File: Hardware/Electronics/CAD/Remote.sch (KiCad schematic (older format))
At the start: 47 parts, among them J1 CONN_01X12, J2 CONN_01X03, J3 CONN_01X05, J4 CONN_01X01, J5 CONN_01X01, J6 CONN_01X24, Q1 AO3418, Q2 Q_NPN_BCE, SW1 SW_DPST_x2, U2 MCP23S17, U3 ESP-12E, U4 LD1117S33CTR

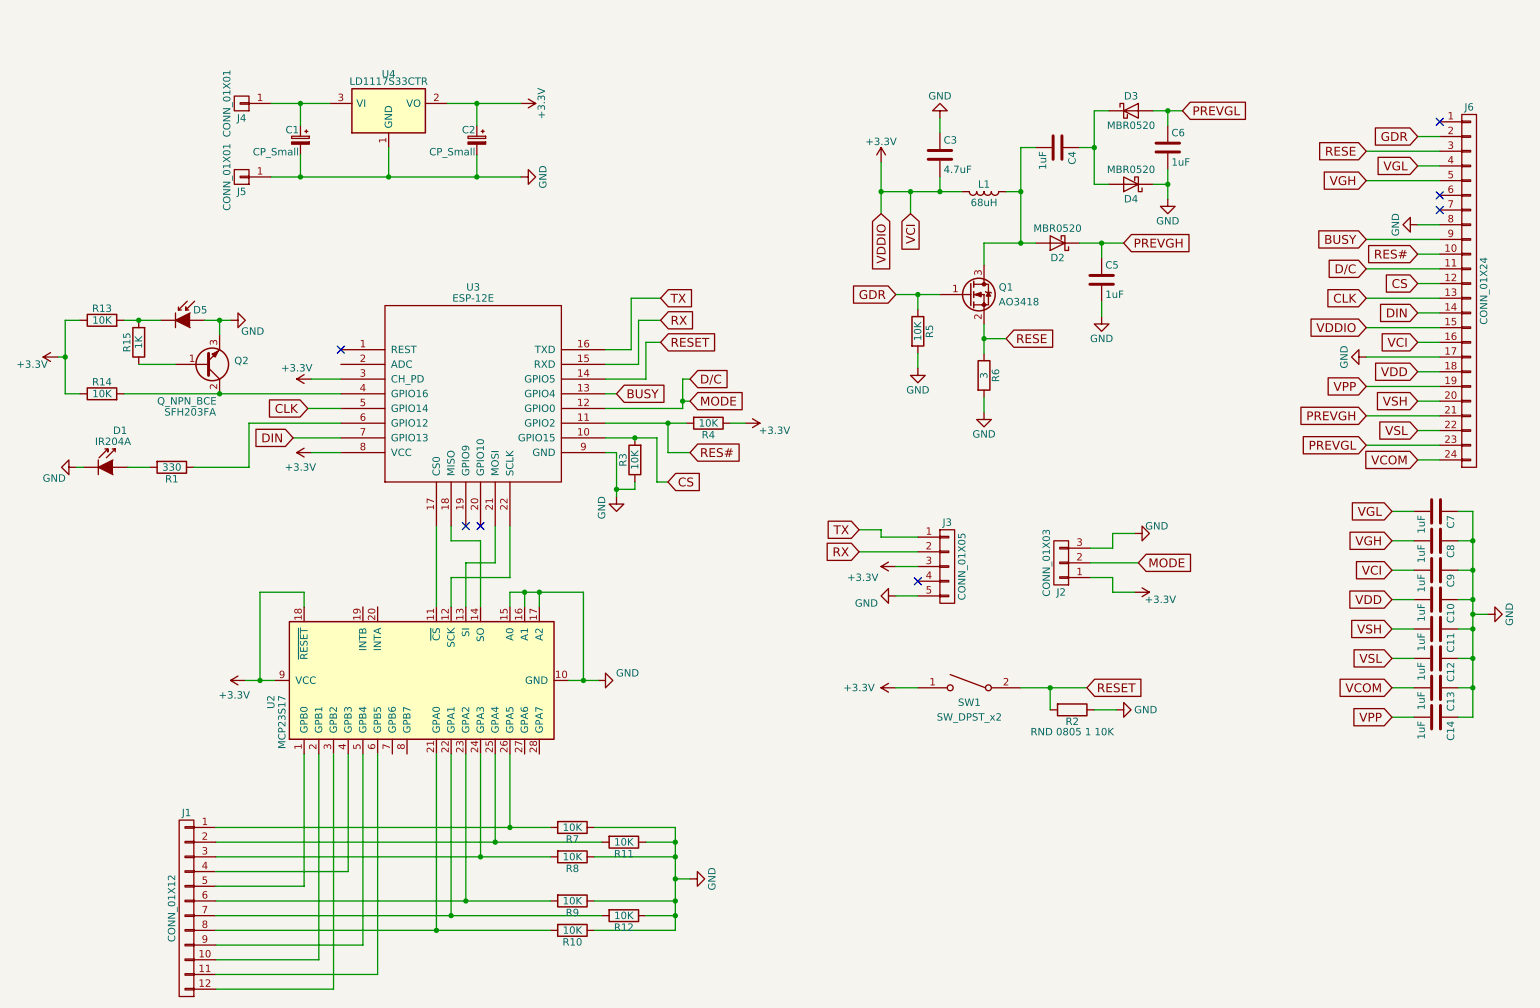
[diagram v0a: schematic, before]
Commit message: update design
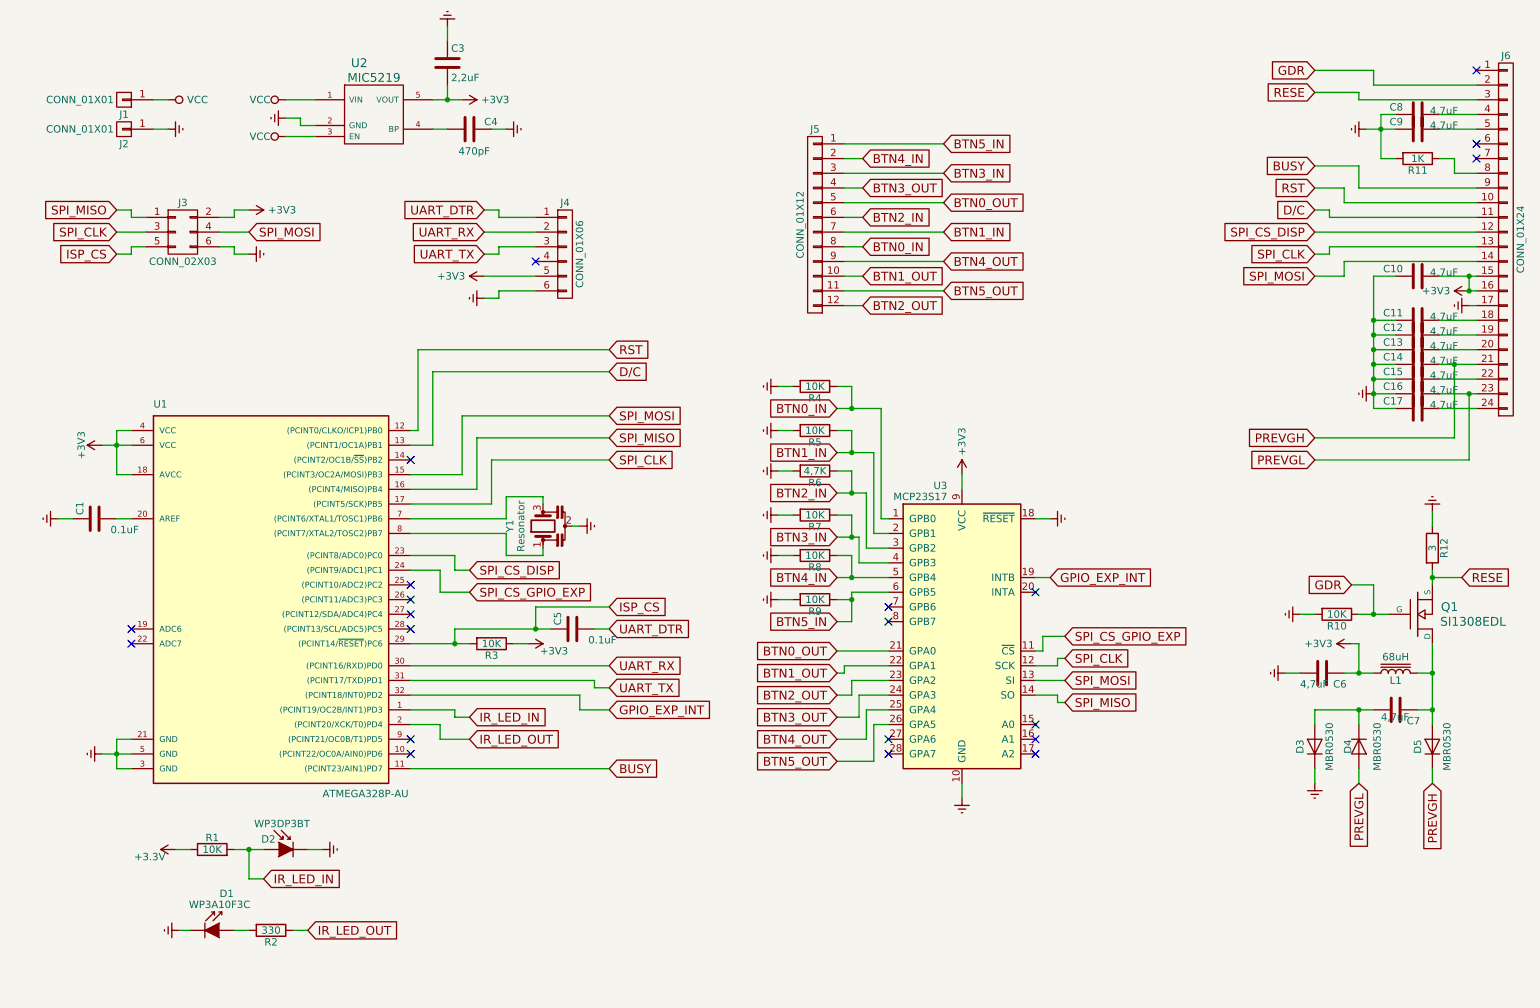
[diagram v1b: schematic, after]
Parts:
- removed C1, C2: CP_Small, Capacitor:CP_8x11.5mm_hor, symbol CP_Small
- removed D2, D3, D4: MBR0520, Diodes_SMD:D_SOD-123, symbol D_Schottky
- removed J2: CONN_01X03, Terminal:Pin_Header_SMD_1x3_Angled_2.54mm, symbol CONN_01X03
- removed J3: CONN_01X05, Terminal:SolderPad_1x5_3.81mm, symbol CONN_01X05
- removed L1: 68uH, Inductors_SMD:L_0805, symbol L
- removed Q1: AO3418, TO_SOT_Packages_SMD:SOT-23, symbol Q_NMOS_GSD
- removed Q2: Q_NPN_BCE, TO_SOT_Packages_SMD:SOT-23, symbol Q_NPN_BCE
- removed R14: 10K, Resistors_SMD:R_0805, symbol R
- removed R15: 1K, Resistors_SMD:R_0805, symbol R
- removed R2: RND 0805 1 10K, Resistors_SMD:R_0805, symbol R
- removed SW1: SW_DPST_x2, Buttons_Switches_SMD:SW_SPST_SKQG, symbol SW_DPST_x2
- removed U2: MCP23S17, Housings_SOIC:SOIC-28W_7.5x17.9mm_Pitch1.27mm, symbol MCP23S17
- removed U3: ESP-12E, ESP8266:ESP-12E_SMD, symbol ESP-12E
- removed U4: LD1117S33CTR, TO_SOT_Packages_SMD:SOT-223, symbol LD1117S33CTR
- added C1: 0.1uF, Capacitors_SMD:C_0805, symbol C
- added C15, C16, C17: 4,7uF, Capacitors_SMD:C_0805, symbol C
- added D3, D4, D5: MBR0530, Diodes_SMD:D_SOD-123, symbol D
- added J3: CONN_02X03, Pin_Headers:Pin_Header_Straight_2x03_Pitch2.54mm, symbol CONN_02X03
- added J4: CONN_01X06, Pin_Headers:Pin_Header_Straight_1x06_Pitch2.54mm, symbol CONN_01X06
- added L1: 68uH, Inductors_SMD:L_1806, symbol L_Core_Iron
- added Q1: SI1308EDL, TO_SOT_Packages_SMD:SOT-323_SC-70, symbol MOSFET_N
- added U1: ATMEGA328P-AU, Housings_QFP:TQFP-32_7x7mm_Pitch0.8mm, symbol ATMEGA328P-AU
- added U2: MIC5219, TO_SOT_Packages_SMD:SOT-23-5, symbol RT9193
- added U3: MCP23S17, SMD_Packages:SOIC-28, symbol MCP23S17
- added Y1: Resonator, Crystals:Resonator_SMD-3pin_7.2x3.0mm, symbol Resonator
- C10, C11, C12, C13, C14, C6, C7, C8, C9: value 1uF -> 4,7uF
- C3: value 4.7uF -> 2,2uF
- C4: value 1uF -> 470pF
- C5: value 1uF -> 0.1uF
- D1: value IR204A -> WP3A10F3C
- D2: renamed from D5; value SFH203FA -> WP3DP3BT
- R11: value 10K -> 1K
- R12: value 10K -> 3
- R6: value 3 -> 4,7K
- renumbered J4 to J1, J5 to J2, J1 to J5, R13 to R1, R1 to R2
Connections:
- net +3V3: now also C10.2, C6.1, R3.1, J3.2 (P2), J4.5 (P5), L1.1, U1.18 (AVCC), U1.4 (VCC), U1.6 (VCC), U2.5 (VOUT), U3.9 (VCC); no longer C9.2, R4.1
- net BUSY: now also U1.11 ((PCINT23/AIN1)PD7)
- net D/C: now also U1.13 ((PCINT1/OC1A)PB1)
- net GDR: now also R10.1, Q1.1 (G); no longer R5.1
- net PREVGH: now also C14.2, D5.1 (K); no longer C5.1
- net PREVGL: now also C16.2, D4.2 (A); no longer C6.1
- net RESE: now also R12.2, Q1.2 (S); no longer R6.1
- net IR_LED_OUT: now reaches R2.1
- net IR_LED_OUT: now also U1.2 ((PCINT20/XCK/T0)PD4)
- net BTN0_OUT: now reaches J5.5 (P5)
- net BTN0_OUT: now also U3.21 (GPA0)
- net BTN1_OUT: now reaches J5.10 (P10)
- net BTN1_OUT: now also U3.22 (GPA1)
- net BTN0_IN: now reaches J5.8 (P8)
- net BTN0_IN: now also R4.1, U3.1 (GPB0); no longer R10.2
- net BTN1_IN: now reaches J5.7 (P7)
- net BTN1_IN: now also R5.1, U3.2 (GPB1); no longer R12.2
- net BTN2_IN: now reaches J5.6 (P6)
- net BTN2_IN: now also R6.1, U3.3 (GPB2); no longer R9.2
- net BTN3_IN: now reaches J5.3 (P3)
- net BTN3_IN: now also R7.1, U3.4 (GPB3); no longer R8.2
- net BTN4_IN: now reaches J5.2 (P2)
- net BTN4_IN: now also R8.1, U3.5 (GPB4); no longer R11.2
- net BTN5_IN: now reaches J5.1 (P1)
- net BTN5_IN: now also R9.1, U3.6 (GPB5); no longer R7.2
- net BTN2_OUT: now reaches J5.12 (P12)
- net BTN2_OUT: now also U3.23 (GPA2)
- net BTN3_OUT: now reaches J5.4 (P4)
- net BTN3_OUT: now also U3.24 (GPA3)
- net BTN4_OUT: now reaches J5.9 (P9)
- net BTN4_OUT: now also U3.25 (GPA4)
- net BTN5_OUT: now reaches J5.11 (P11)
- net BTN5_OUT: now also U3.26 (GPA5)
- net VCC: now reaches J1.1 (P1)
- net VCC: now also U2.1 (VIN), U2.3 (EN)
- net at C4.2: now also U2.4 (BP)
- net Earth: now reaches C4.1
- net Earth: now also C10.1, C11.1, C12.1, C13.1, C14.1, C3.1, C6.2, C8.1, C9.1, D1.1 (K), D2.1 (K), J2.1 (P1), J6.17 (P17), R10.2, R11.2, R12.1, R4.2, R5.2, R6.2, R7.2, R8.2, R9.2, C1.1, C15.1, C16.1, C17.1, D3.1 (K), J3.6 (P6), J4.6 (P6), U1.21 (GND), U1.3 (GND), U1.5 (GND), U2.2 (GND), U3.10 (GND), U3.18 (~RESET), Y1.2
- net IR_LED_IN: now reaches R1.2
- net IR_LED_IN: now also D2.2 (A), U1.1 ((PCINT19/OC2B/INT1)PD3); no longer D2.1 (K)
- net CLK renamed SPI_CLK
- net SPI_CLK: now also J3.3 (P3), U1.17 ((PCINT5/SCK)PB5), U3.12 (SCK)
- net CS renamed ISP_CS
- net ISP_CS: now also C5.1, J3.5 (P5), U1.29 ((PCINT14/~RESET~)PC6); no longer J6.12 (P12)
- net DIN renamed SPI_MOSI
- net SPI_MOSI: now also J3.4 (P4), U1.15 ((PCINT3/OC2A/MOSI)PB3), U3.13 (SI)
- removed net GND: C10.1, C11.1, C12.1, C13.1, C14.1, C3.1, C5.2, C6.2, C7.1, C8.1, C9.1, D1.1 (K), D2.2 (A), J2.1 (P1), J6.17 (P17), J6.8 (P8), R10.1, R11.1, R12.1, R3.1, R5.2, R6.2, R7.1, R8.1, R9.1
- net RES# renamed RST
- net RST: now also U1.12 ((PCINT0/CLKO/ICP1)PB0); no longer R4.2
- net VCOM: no longer names the net of C13.2
- net VCOM: now also J6.20 (P20); no longer J6.24 (P24)
- net VDD: no longer names the net of J6.18 (P18)
- net VDD: now also C11.2; no longer C10.2
- net VGH: no longer names the net of C8.2
- net VGH: now also J6.4 (P4); no longer J6.5 (P5)
- net VGL: no longer names the net of C7.2
- net VGL: now also D3.2 (A), D4.1 (K); no longer J6.4 (P4)
- net VPP: no longer names the net of J6.19 (P19)
- net VPP: now also C12.2; no longer C14.2
- removed net VSH: C11.2, J6.20 (P20)
- net VSL: no longer names the net of J6.22 (P22)
- net VSL: now also C15.2; no longer C12.2
- new net: C17.2, J6.24 (P24)
- new net: C9.2, J6.5 (P5)
- new net: J6.8 (P8), R11.1
- new net: C7.1, D5.2 (A), L1.2, Q1.3 (D)
- new net: C1.2, U1.20 (AREF)
- new net: U1.7 ((PCINT6/XTAL1/TOSC1)PB6), Y1.3
- new net: U1.8 ((PCINT7/XTAL2/TOSC2)PB7), Y1.1
- new net GPIO_EXP_INT: U1.32 ((PCINT18/INT0)PD2), U3.19 (INTB)
- new net SPI_CS_DISP: J6.12 (P12), U1.23 ((PCINT8/ADC0)PC0)
- new net SPI_CS_GPIO_EXP: U1.24 ((PCINT9/ADC1)PC1), U3.11 (~CS)
- new net SPI_MISO: J3.1 (P1), U1.16 ((PCINT4/MISO)PB4), U3.14 (SO)
- new net UART_DTR: C5.2, J4.1 (P1)
- new net UART_RX: J4.2 (P2), U1.30 ((PCINT16/RXD)PD0)
- new net UART_TX: J4.3 (P3), U1.31 ((PCINT17/TXD)PD1)
- no-connect marks 7 -> 21
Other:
- moved on the sheet: D1, D2, J1, J2, J5, R1, R2
